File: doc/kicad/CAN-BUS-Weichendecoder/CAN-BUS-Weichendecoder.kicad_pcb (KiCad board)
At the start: 2 copper layers, 25 parts, among them J1 RJ45_LED_Shielded, J2 RJ45_Shielded, K1 HFD2_005-S-L2-D, U1 ULN2803A, U2 ULN2803A, U3 PCF8574, U4 PCF8574, U5 PCF8574, U6 ULN2803A, U7 ULN2803A, U8 ULN2803A

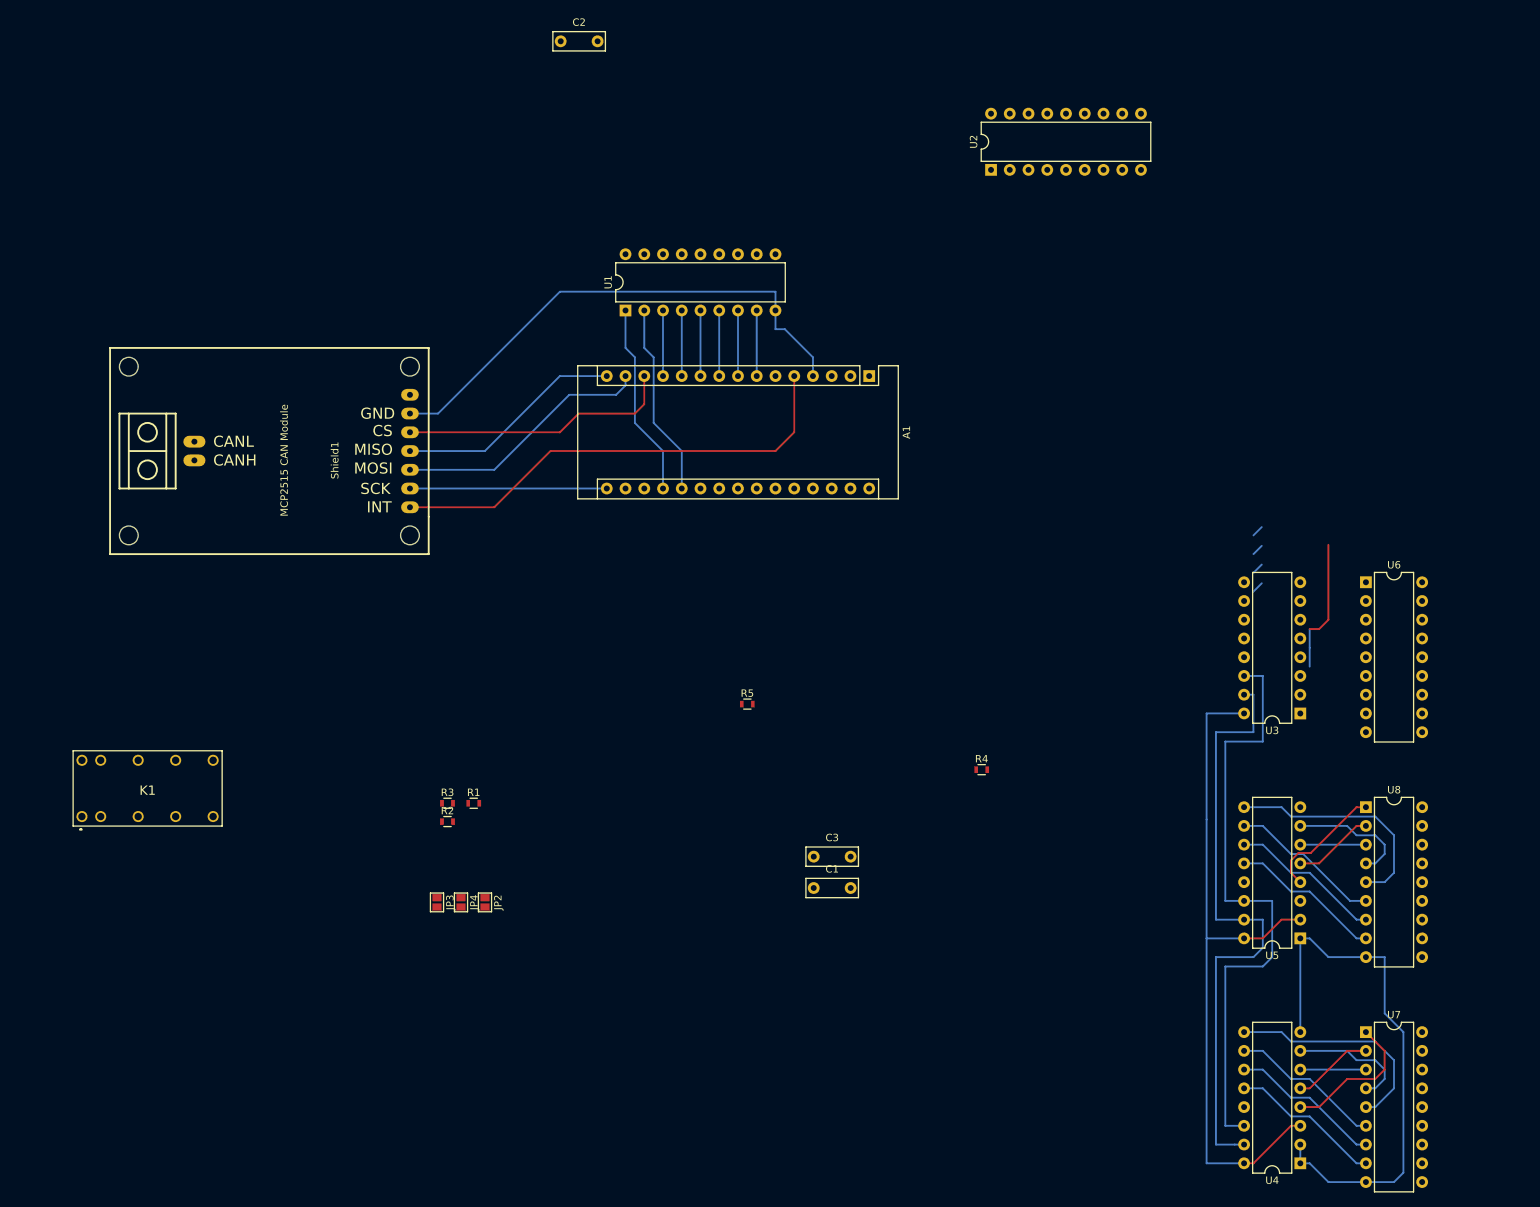
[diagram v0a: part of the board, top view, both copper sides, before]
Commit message: Aktueller Stand
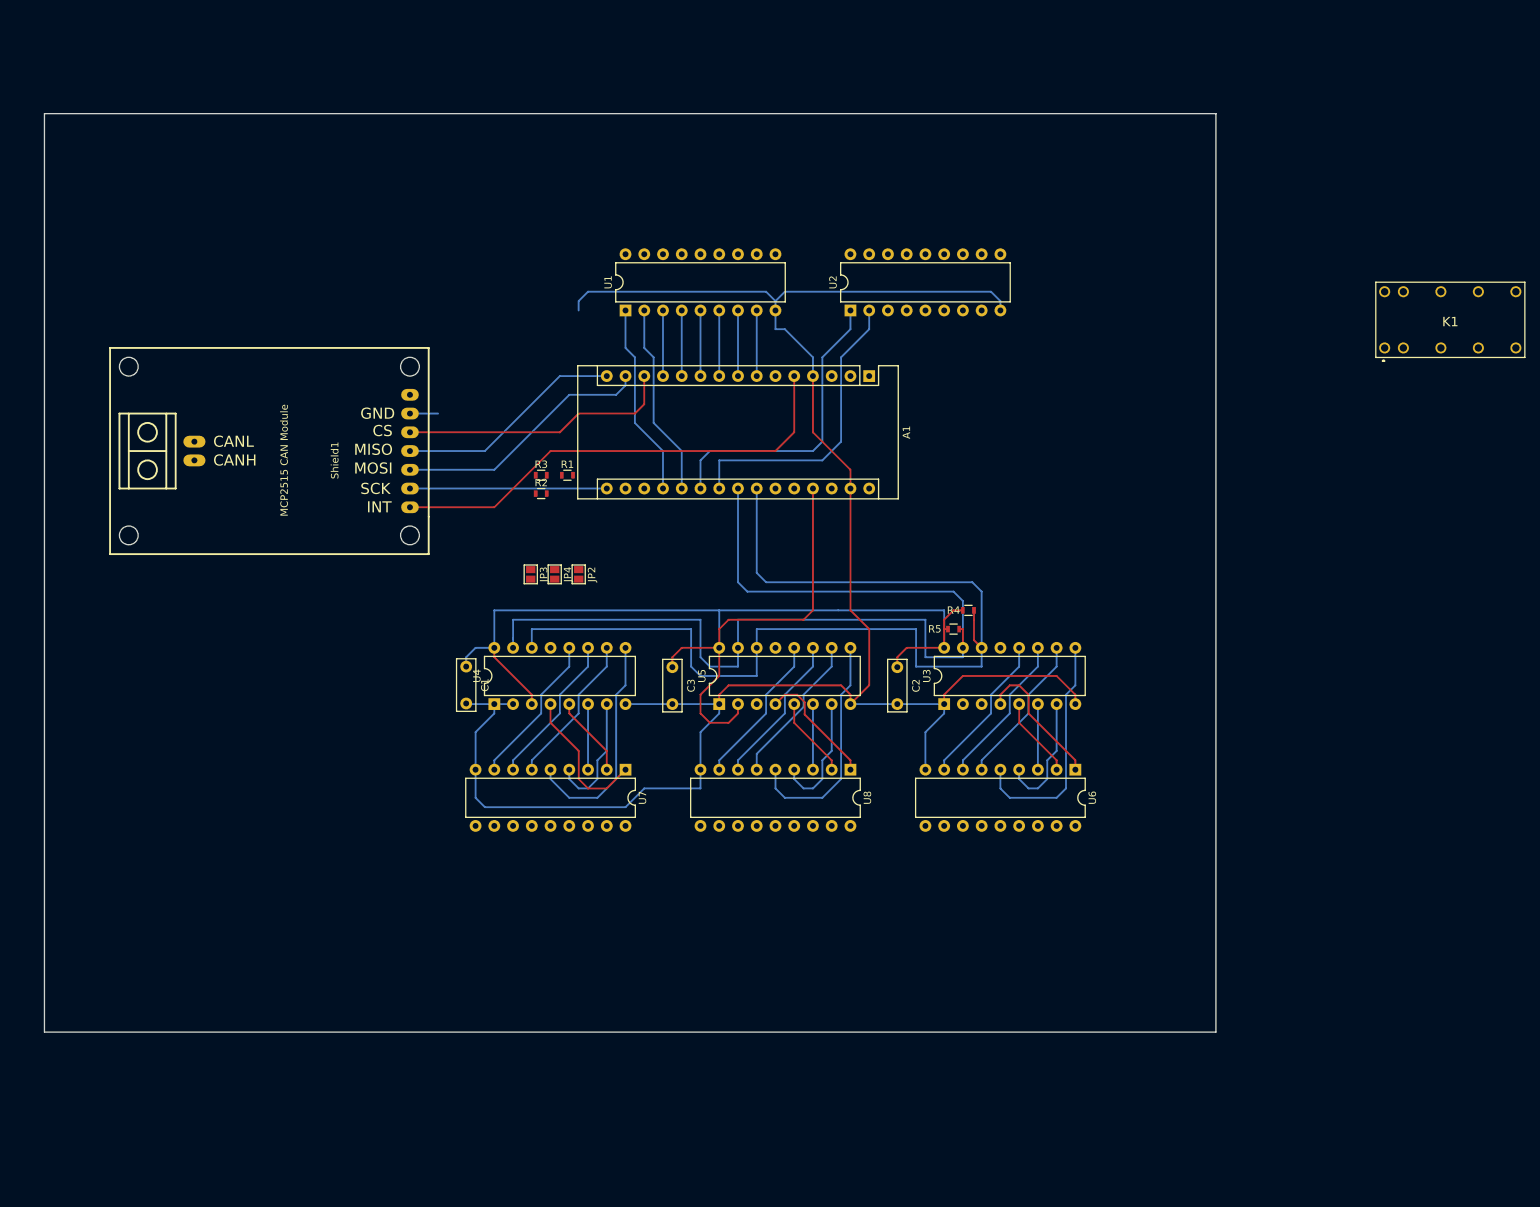
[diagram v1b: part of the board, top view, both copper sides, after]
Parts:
- moved K1 187.6 mm to (201.9, 52.1)
- moved U4 125.7 mm to (81.3, 100.3), turned to 90 degrees
- moved U7 106.4 mm to (99.1, 109.2), turned to 270 degrees
- moved C2 96.3 mm to (135.9, 95.3), turned to 270 degrees
- moved U5 84.9 mm to (111.8, 100.3), turned to 90 degrees
- moved U8 70.0 mm to (129.5, 109.2), turned to 270 degrees
- moved C1 55.8 mm to (77.5, 95.2), turned to 270 degrees
- moved U3 48.3 mm to (142.2, 100.3), turned to 90 degrees
- moved U6 46.9 mm to (160.0, 109.2), turned to 270 degrees
- moved JP2 46.2 mm to (92.7, 82.8)
- moved JP3 46.2 mm to (86.2, 82.8)
- moved JP4 46.2 mm to (89.5, 82.8)
- moved R2 46.2 mm to (87.6, 71.8)
- moved R1 46.2 mm to (91.2, 69.3)
- moved R3 46.2 mm to (87.6, 69.3)
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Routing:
- net GND: track 212.0 -> 320.7 mm
- net +5V: track 94.6 -> 165.5 mm
- net Net-(A1-Pad24): track 83.1 -> 139.2 mm
- net Net-(A1-Pad23): track 83.1 -> 136.7 mm
- net Net-(A1-Pad22): track 0.00 -> 40.7 mm
- net Net-(A1-Pad21): track 0.00 -> 40.7 mm
- net Net-(U3-Pad9): track 1.59 -> 32.1 mm
- net Net-(U3-Pad12): track 1.59 -> 20.7 mm
- net Net-(U3-Pad11): track 1.59 -> 20.7 mm
- net Net-(U3-Pad10): track 1.59 -> 20.7 mm
- net Net-(U3-Pad4): track 0.00 -> 18.9 mm
- net Net-(U3-Pad7): track 0.00 -> 16.8 mm
- net Net-(U3-Pad5): track 0.00 -> 11.0 mm
- net Net-(U3-Pad6): track 0.00 -> 8.89 mm
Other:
- board outline added: 158.8 x 124.5 mm
